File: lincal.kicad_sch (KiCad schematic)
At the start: 0 parts

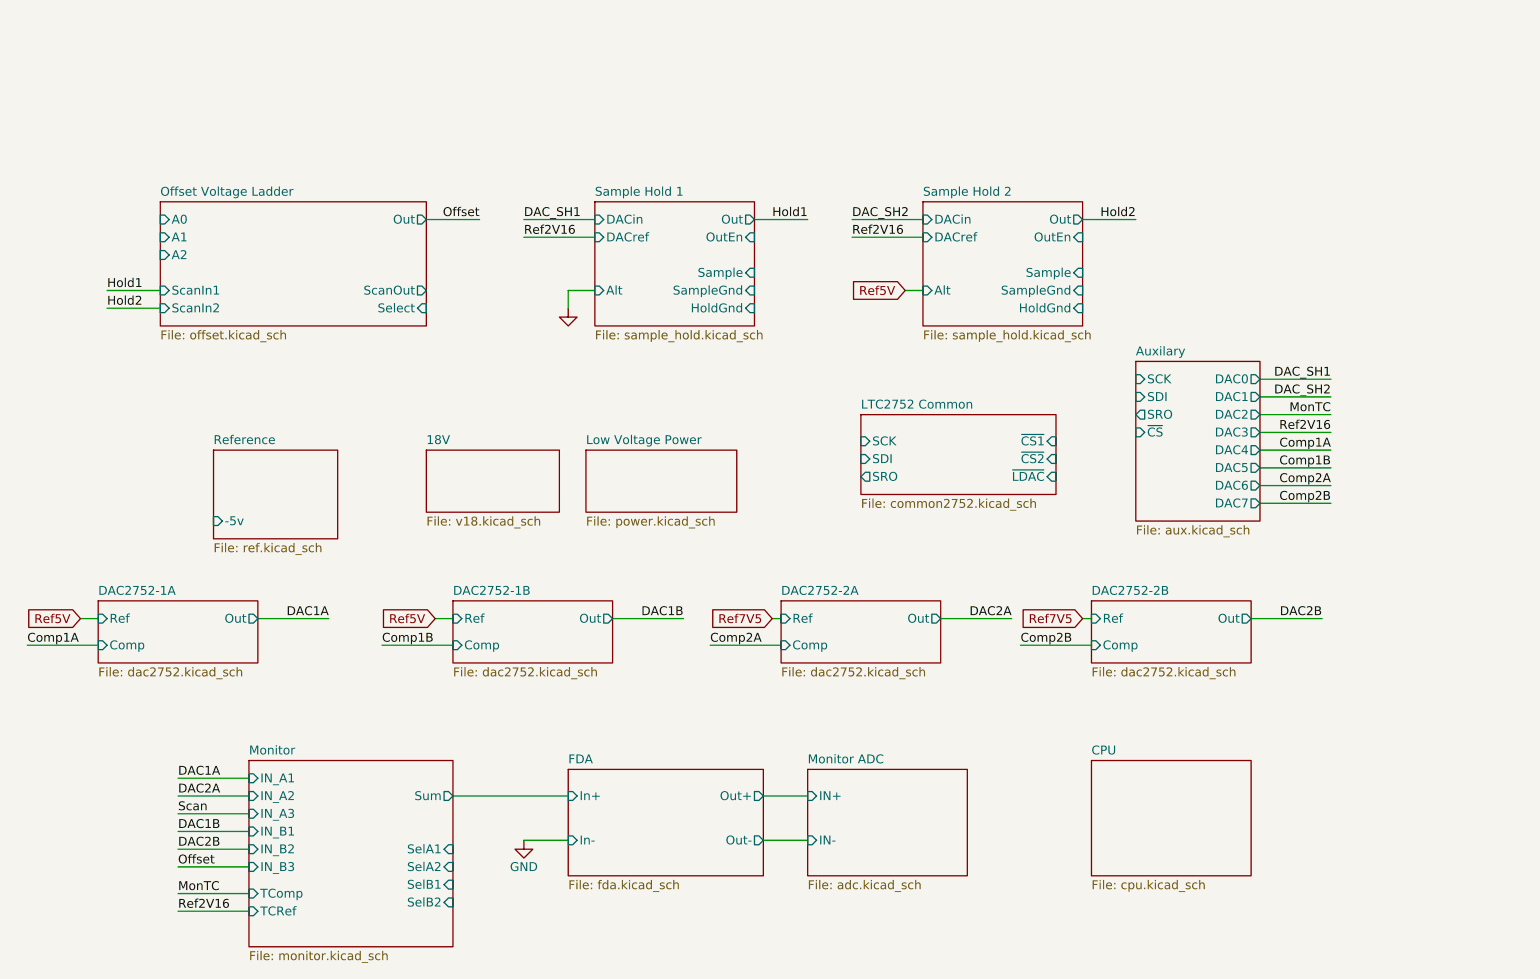
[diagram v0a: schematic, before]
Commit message: Schematic complete, maybe
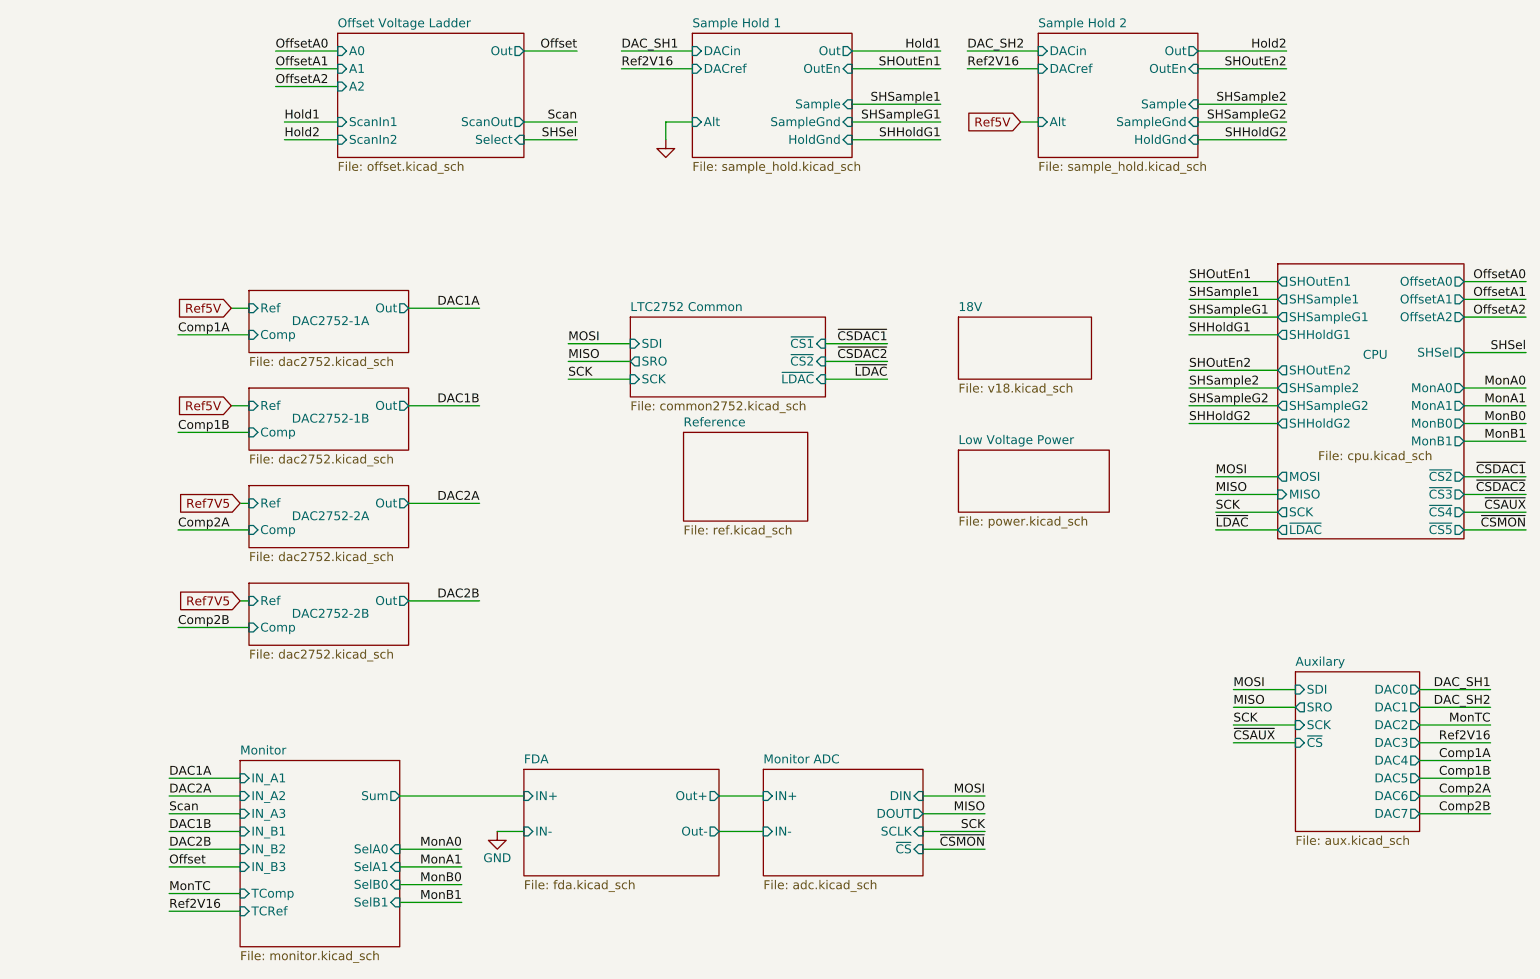
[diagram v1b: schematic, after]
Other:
- sheet CPU ports: added MISO, MOSI, MonA0, MonA1, MonB0, MonB1, OffsetA0, OffsetA1, OffsetA2, SCK, SHHoldG1, SHHoldG2, SHOutEn1, SHOutEn2, SHSample1, SHSample2, SHSampleG1, SHSampleG2, SHSel, ~{CS2}, ~{CS3}, ~{CS4}, ~{CS5}, ~{LDAC}; removed none
- sheet FDA ports: added IN+, IN-; removed In+, In-
- sheet Monitor ports: added SelA0, SelB0; removed SelA2, SelB2
- sheet Monitor ADC ports: added DIN, DOUT, SCLK, ~{CS}; removed none
- sheet Reference ports: added none; removed -5v

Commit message: Everything assigned except for wierd shit.
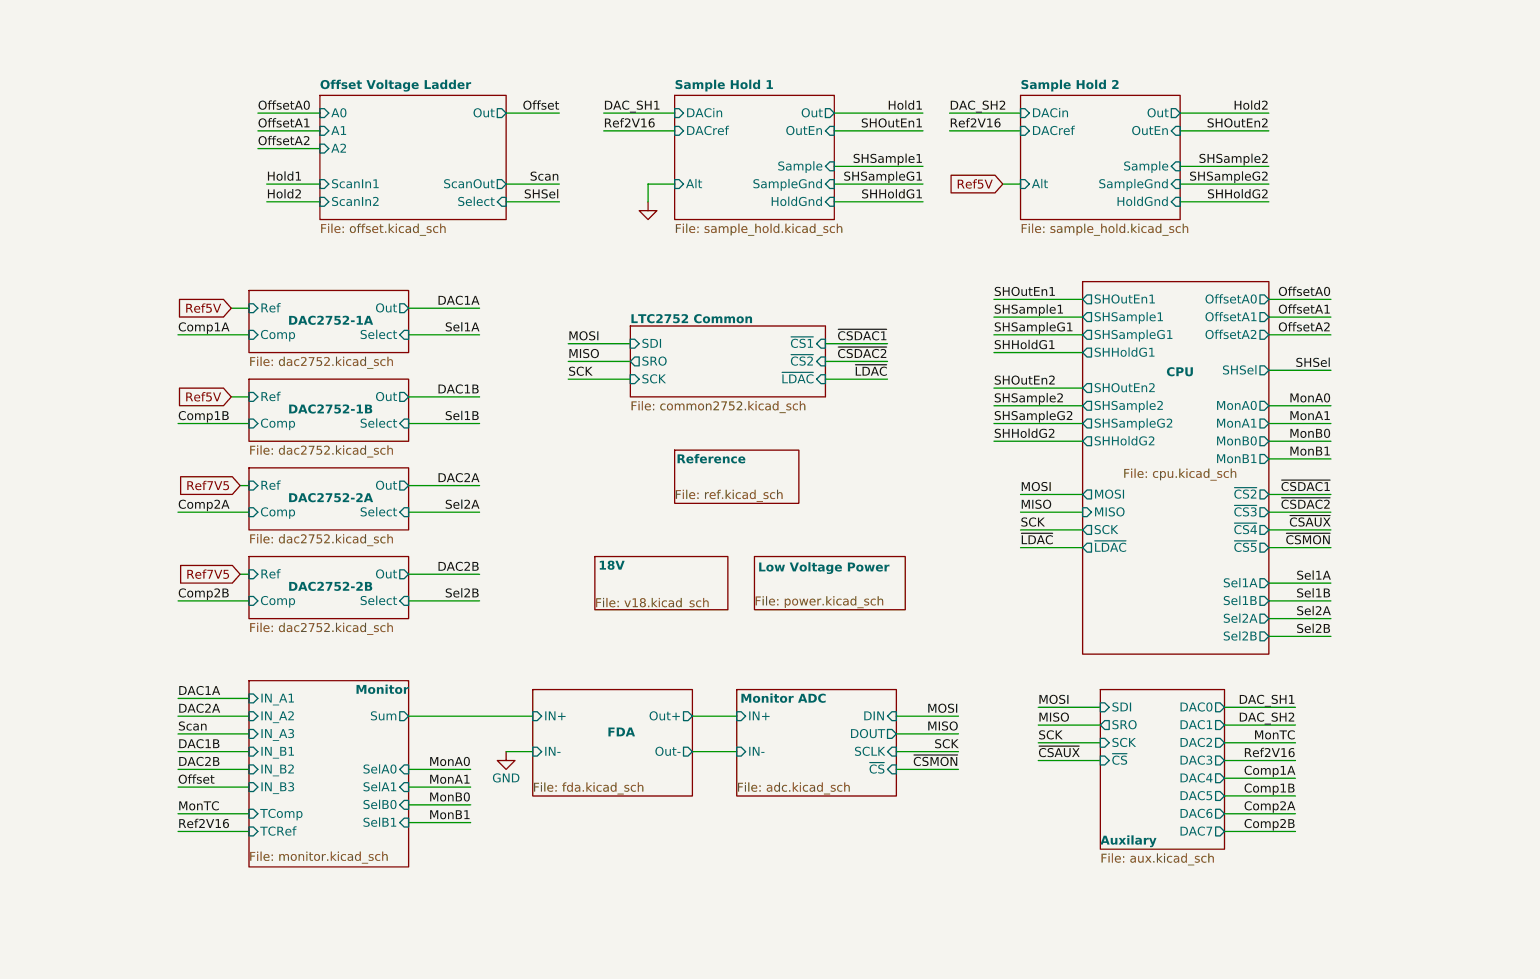
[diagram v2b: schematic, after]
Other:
- sheet CPU ports: added Sel1A, Sel1B, Sel2A, Sel2B; removed none
- sheet DAC2752-1A ports: added Select; removed none
- sheet DAC2752-1B ports: added Select; removed none
- sheet DAC2752-2A ports: added Select; removed none
- sheet DAC2752-2B ports: added Select; removed none
